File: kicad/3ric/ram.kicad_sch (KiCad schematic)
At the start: 7 parts, among them M2_VBUS_LOW1 74LS245, M3_VBUS_HIGH1 74LS245

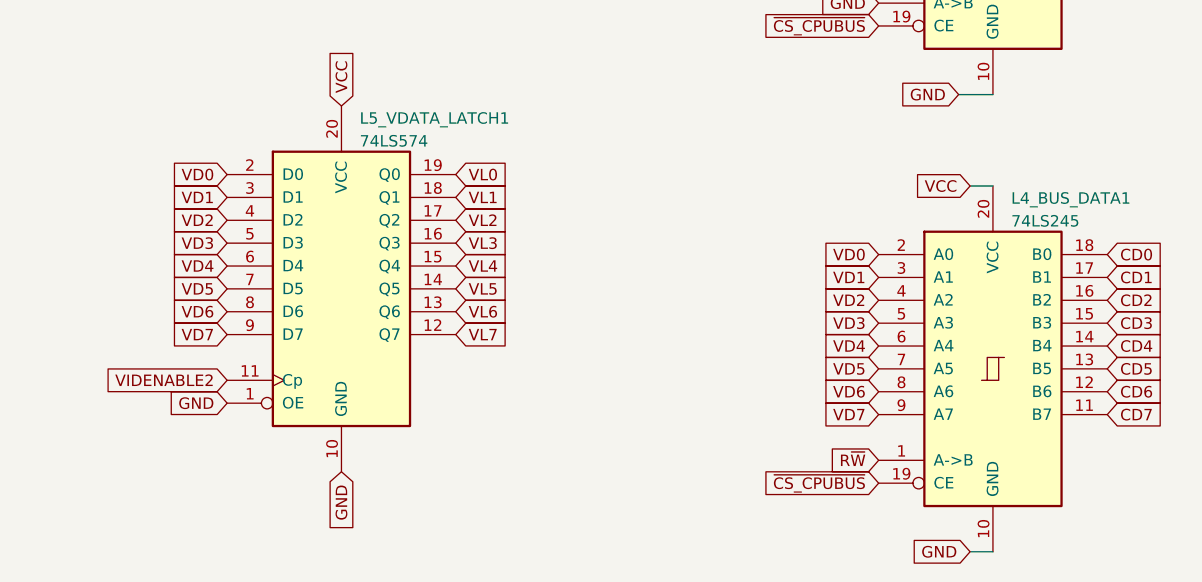
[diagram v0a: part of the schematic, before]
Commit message: pcb layout continued
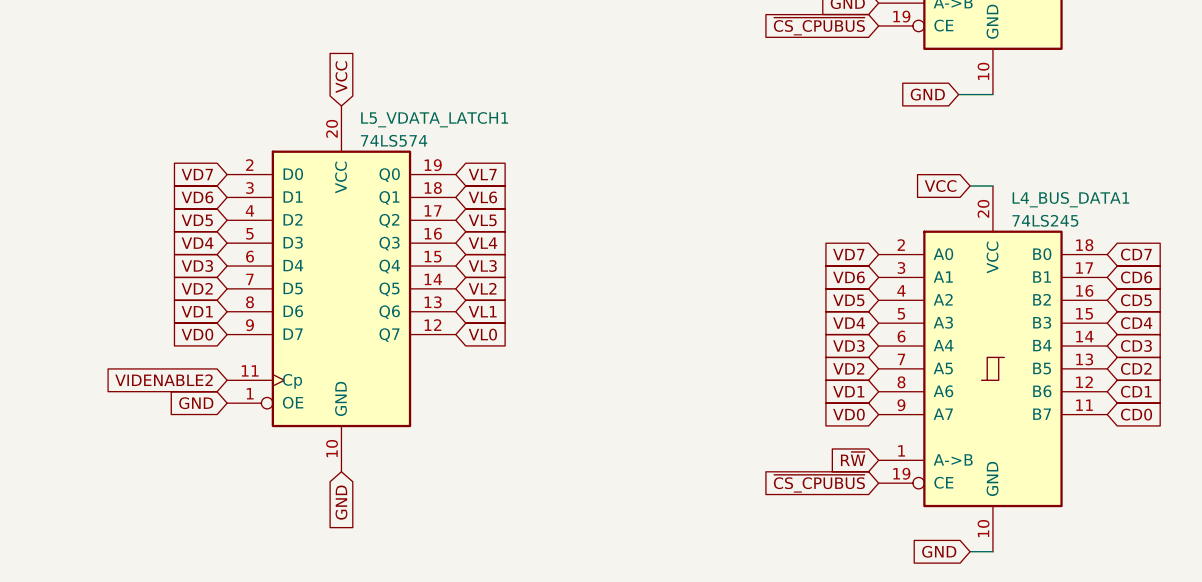
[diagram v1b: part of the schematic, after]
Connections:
- net CD0: now also L4_BUS_DATA1.11 (B7); no longer L4_BUS_DATA1.18 (B0)
- net CD1: now also L4_BUS_DATA1.12 (B6); no longer L4_BUS_DATA1.17 (B1)
- net CD2: now also L4_BUS_DATA1.13 (B5); no longer L4_BUS_DATA1.16 (B2)
- net CD3: now also L4_BUS_DATA1.14 (B4); no longer L4_BUS_DATA1.15 (B3)
- net CD4: now also L4_BUS_DATA1.15 (B3); no longer L4_BUS_DATA1.14 (B4)
- net CD5: now also L4_BUS_DATA1.16 (B2); no longer L4_BUS_DATA1.13 (B5)
- net CD6: now also L4_BUS_DATA1.17 (B1); no longer L4_BUS_DATA1.12 (B6)
- net CD7: now also L4_BUS_DATA1.18 (B0); no longer L4_BUS_DATA1.11 (B7)
- net VD0: now also L4_BUS_DATA1.9 (A7), L5_VDATA_LATCH1.9 (D7); no longer L4_BUS_DATA1.2 (A0), L5_VDATA_LATCH1.2 (D0)
- net VD1: now also L4_BUS_DATA1.8 (A6), L5_VDATA_LATCH1.8 (D6); no longer L4_BUS_DATA1.3 (A1), L5_VDATA_LATCH1.3 (D1)
- net VD2: now also L4_BUS_DATA1.7 (A5), L5_VDATA_LATCH1.7 (D5); no longer L4_BUS_DATA1.4 (A2), L5_VDATA_LATCH1.4 (D2)
- net VD3: now also L4_BUS_DATA1.6 (A4), L5_VDATA_LATCH1.6 (D4); no longer L4_BUS_DATA1.5 (A3), L5_VDATA_LATCH1.5 (D3)
- net VD4: now also L4_BUS_DATA1.5 (A3), L5_VDATA_LATCH1.5 (D3); no longer L4_BUS_DATA1.6 (A4), L5_VDATA_LATCH1.6 (D4)
- net VD5: now also L4_BUS_DATA1.4 (A2), L5_VDATA_LATCH1.4 (D2); no longer L4_BUS_DATA1.7 (A5), L5_VDATA_LATCH1.7 (D5)
- net VD6: now also L4_BUS_DATA1.3 (A1), L5_VDATA_LATCH1.3 (D1); no longer L4_BUS_DATA1.8 (A6), L5_VDATA_LATCH1.8 (D6)
- net VD7: now also L4_BUS_DATA1.2 (A0), L5_VDATA_LATCH1.2 (D0); no longer L4_BUS_DATA1.9 (A7), L5_VDATA_LATCH1.9 (D7)
- net VL0: now also L5_VDATA_LATCH1.12 (Q7); no longer L5_VDATA_LATCH1.19 (Q0)
- net VL1: now also L5_VDATA_LATCH1.13 (Q6); no longer L5_VDATA_LATCH1.18 (Q1)
- net VL2: now also L5_VDATA_LATCH1.14 (Q5); no longer L5_VDATA_LATCH1.17 (Q2)
- net VL3: now also L5_VDATA_LATCH1.15 (Q4); no longer L5_VDATA_LATCH1.16 (Q3)
- net VL4: now also L5_VDATA_LATCH1.16 (Q3); no longer L5_VDATA_LATCH1.15 (Q4)
- net VL5: now also L5_VDATA_LATCH1.17 (Q2); no longer L5_VDATA_LATCH1.14 (Q5)
- net VL6: now also L5_VDATA_LATCH1.18 (Q1); no longer L5_VDATA_LATCH1.13 (Q6)
- net VL7: now also L5_VDATA_LATCH1.19 (Q0); no longer L5_VDATA_LATCH1.12 (Q7)
